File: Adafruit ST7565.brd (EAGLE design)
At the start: 58.1 x 48.2 mm, 19 parts, among them IC1 4050D, IC2 L4931D-GNDPIN7, Q3 2N7002, Q4 2N7002, SW1 ROTARTY_ENCODER, U1 SD_CARD_SOCKET

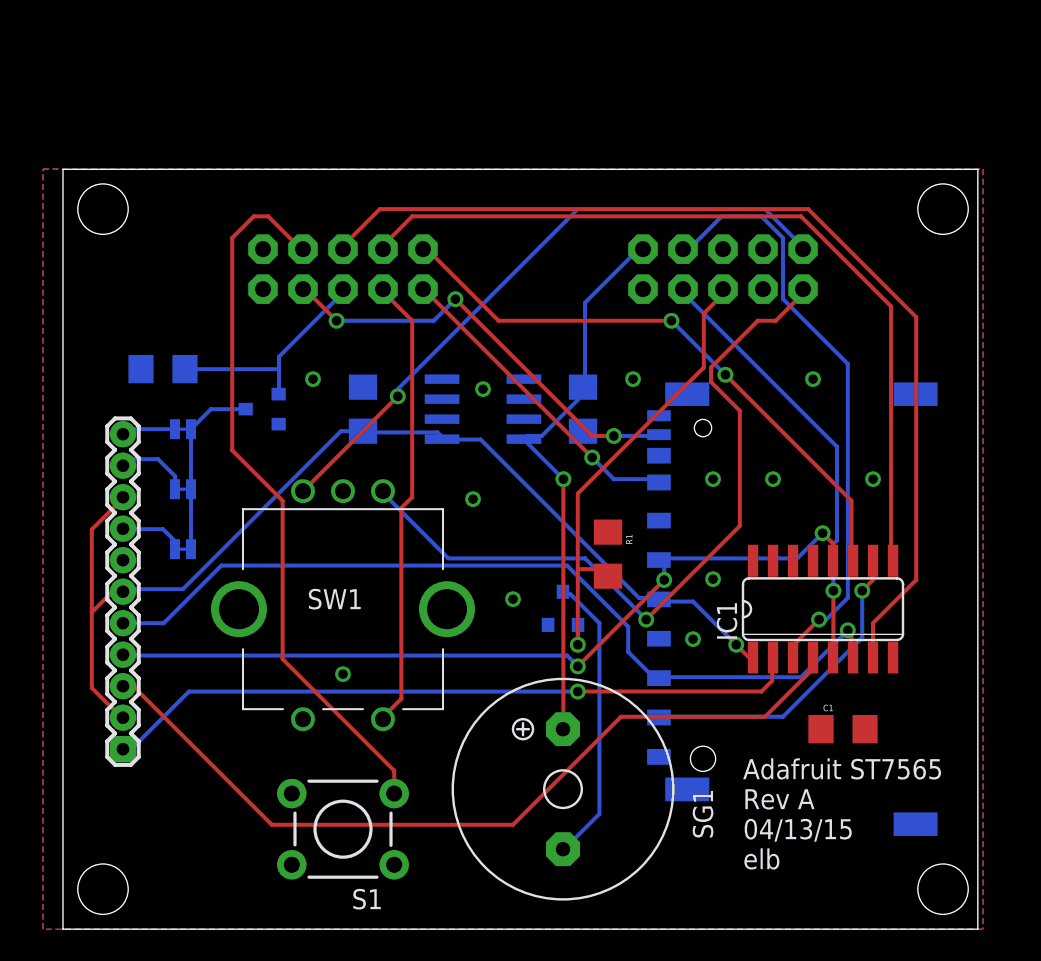
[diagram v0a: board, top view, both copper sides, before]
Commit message: Rev B
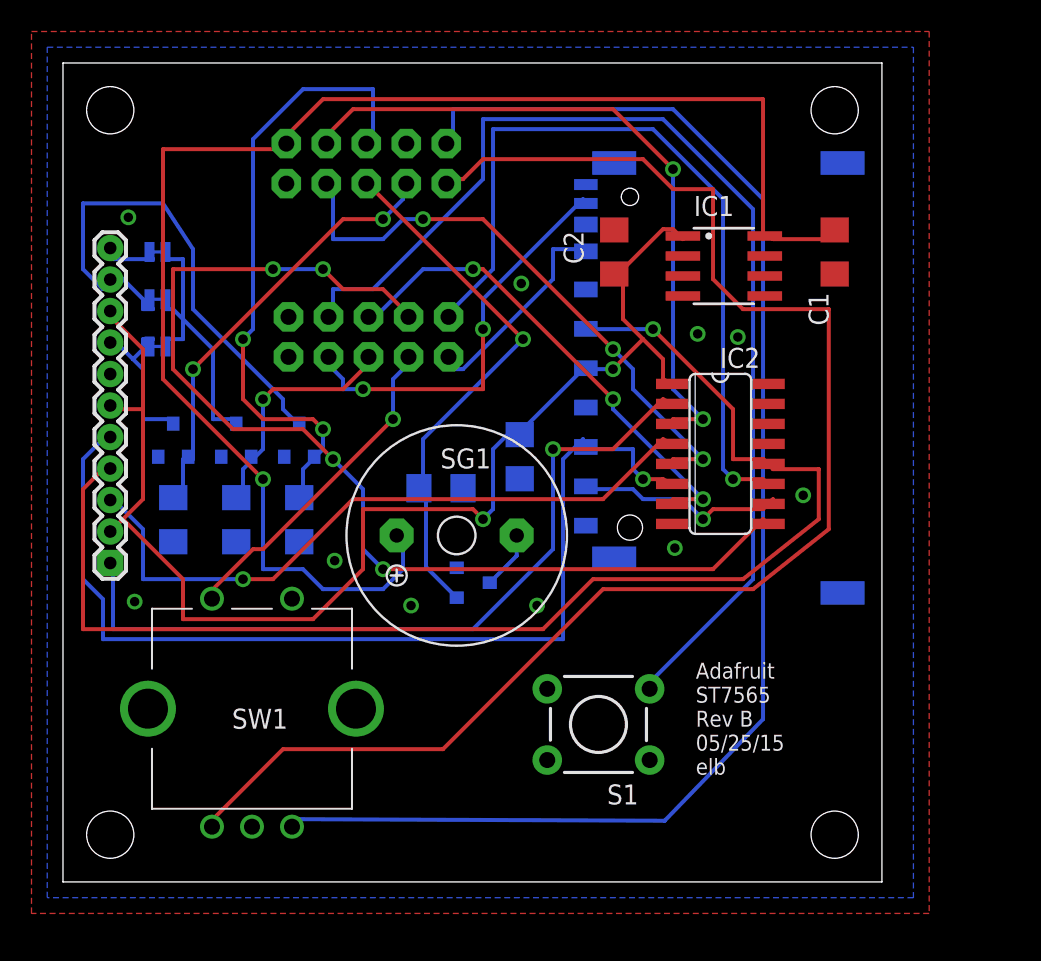
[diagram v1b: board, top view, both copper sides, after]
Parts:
- removed BLUE: Blue, SparkFun-Passives:PAD-JUMPER-2-NC_BY_TRACE_YES_SILK
- removed C4: 2.2uF, SparkFun-Passives:1206
- removed GREEN: Green, SparkFun-Passives:PAD-JUMPER-2-NC_BY_TRACE_YES_SILK
- removed RED: Red, SparkFun-Passives:PAD-JUMPER-2-NC_BY_TRACE_YES_SILK
- removed U$1: 1X11_2MM, elb:1X11_2MM
- added B: Blue, SparkFun-Passives:PAD-JUMPER-2-NC_BY_TRACE_YES_SILK
- added C2: 2.2uF, SparkFun-Passives:1206
- added G: Green, SparkFun-Passives:PAD-JUMPER-2-NC_BY_TRACE_YES_SILK
- added JP3: 1X11_2MM, elb:1X11_2MM
- added Q1, Q2: 2N7002, SparkFun-DiscreteSemi:SOT23-3
- added R: Red, SparkFun-Passives:PAD-JUMPER-2-NC_BY_TRACE_YES_SILK
- added R3, R4: 4.7k, SparkFun-Passives:1206
- C1: value 1 uF -> 0.1uF
- C3: value 0.1uF -> 1 uF
- IC1: value 4050D -> L4931D; device 40xx:SO16 -> v-reg-3:SO08
- IC2: value L4931D-GNDPIN7 -> 4050D; device v-reg-3:SO08 -> 40xx:SO16
- moved C1 30.3 mm to (49.0, 43.0), turned to 270 degrees
- moved JP1 23.6 mm to (19.3, 48.6)
- moved IC1 22.7 mm to (42.0, 42.1), turned to 270 degrees
- moved Q3 19.9 mm to (15.0, 31.0)
- moved S1 17.5 mm to (34.0, 13.0)
- moved SG1 17.5 mm to (25.0, 25.0), turned to 180 degrees
- moved U1 15.4 mm to (36.0, 35.0)
- moved IC2 15.3 mm to (41.7, 30.2), flipped to the top, turned to 270 degrees
- moved R1 11.4 mm to (24.0, 28.0), flipped to the bottom, turned to 0 degrees
- moved R2 10.6 mm to (11.0, 26.0), turned to 90 degrees
- moved SW1 8.56 mm to (12.0, 14.0), turned to 270 degrees
- moved Q4 6.05 mm to (7.00, 31.0), turned to 0 degrees
- moved C3 5.03 mm to (29.0, 30.0)
- moved JP2 4.60 mm to (19.4, 37.6)
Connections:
- removed net N$6: GREEN.2, U$1.10
- removed net N$7: BLUE.2, U$1.11
- new net D17: JP1.8, Q4.1, R4.2
- new net D25: JP1.5, Q3.1, R3.2
- new net N$3: B.2, JP3.11
- new net N$4: G.2, JP3.10, Q3.3
- net +3.3V: now also C2.1, C3.1, JP3.2, JP3.6, JP3.9; no longer C1.1, C4.1, U$1.2, U$1.6, U$1.9
- net +5V: now also C1.1, IC1.8; no longer C3.1, IC2.8
- net D23: now also Q1.1; no longer Q3.1
- net D27: now also IC2.5; no longer IC1.5
- net D29: now also IC2.3; no longer IC1.3
- net D33: now also Q2.1; no longer Q4.1
- net D51: now also IC2.7; no longer IC1.7
- net D52: now also IC2.11; no longer IC1.11
- net D53: now also IC2.9; no longer IC1.9
- net GND: now also C2.2, IC1.7, IC2.14, IC2.8, JP2.2, JP3.7, Q1.2, Q2.2, R3.1, R4.1; no longer C4.2, IC1.14, IC1.8, IC2.7, U$1.7
- net LCD_A0: now also IC2.4, JP3.3; no longer IC1.4, U$1.3
- net LCD_CS: now also IC2.2, JP3.1; no longer IC1.2, U$1.1
- net MOSI: now also IC2.6, JP3.5; no longer IC1.6, U$1.5
- net N$1: now also Q1.3; no longer Q3.3
- net N$2: now also B.1, G.1, Q2.3, R.1; no longer BLUE.1, GREEN.1, Q4.3, RED.1
- net N$5: now also JP3.8, Q4.3, R.2; no longer RED.2, U$1.8
- net SCLK: now also IC2.12, JP3.4; no longer IC1.12, U$1.4
- net SD_CS: now also IC2.10; no longer IC1.10
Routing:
- net +5V: track 35.5 -> 95.6 mm
- net D35: track 40.7 -> 90.5 mm, vias 1 -> 0
- net D37: track 47.5 -> 93.1 mm, vias 1 -> 0
- net D25: track 0.00 -> 40.4 mm, vias 0 -> 2
- net N$4: track 0.00 -> 35.2 mm
- net SCLK: track 51.8 -> 84.5 mm, vias 3 -> 1
- net D51: track 63.4 -> 31.2 mm, vias 0 -> 3
- net D17: track 0.00 -> 28.0 mm, vias 0 -> 2
- net D41: track 45.5 -> 70.7 mm
- net D53: track 52.1 -> 69.4 mm, vias 0 -> 4
- net N$1: track 18.6 -> 3.71 mm
- net +3.3V: track 68.5 -> 82.4 mm, vias 1 -> 2
- net D52: track 37.8 -> 49.9 mm, vias 2 -> 1
- net MOSI: track 54.7 -> 64.3 mm
- net D27: track 27.6 -> 37.0 mm, vias 1 -> 3
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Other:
- board size 58.1 x 48.2 mm -> 52 x 52 mm
- board text added: "Adafruit ST7565 Rev B 05/25/15 elb"
- board text removed: "Adafruit ST7565 Rev A 04/13/15 elb"
